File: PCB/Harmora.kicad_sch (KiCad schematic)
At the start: 14 parts, among them U14 ATmega328p-AU, U17 128x64 2.42 inc, Y1 16Mhz

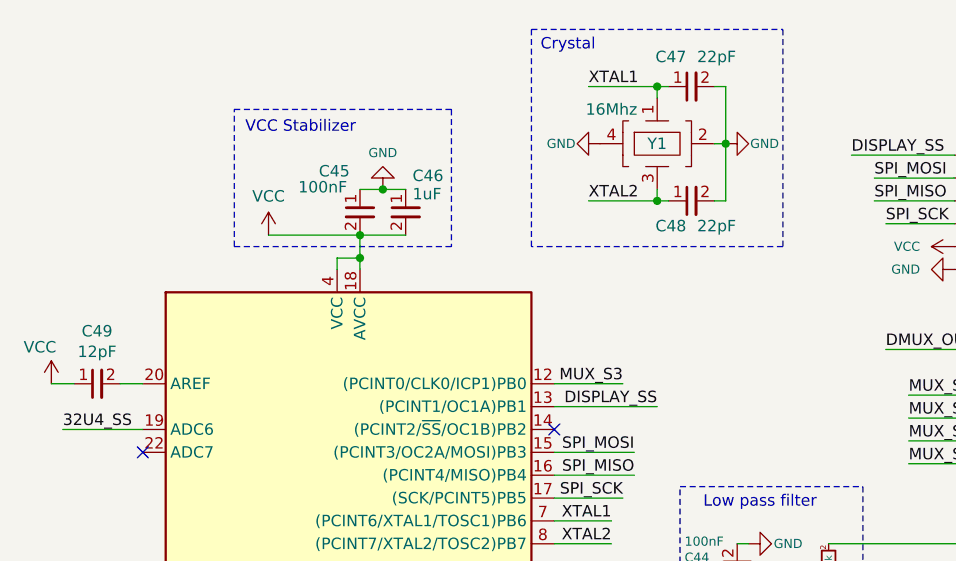
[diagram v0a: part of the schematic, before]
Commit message: new schematics
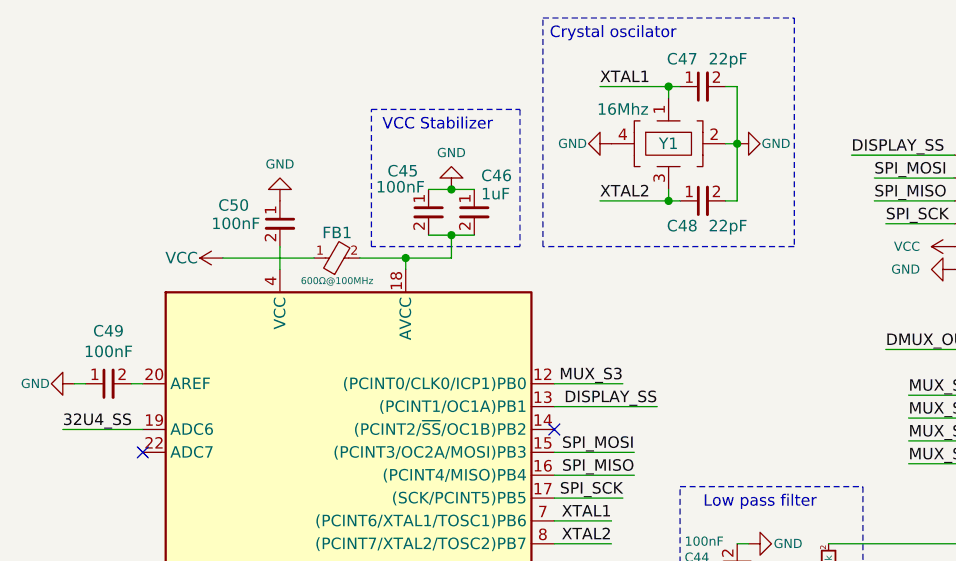
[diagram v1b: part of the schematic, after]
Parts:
- added C50: 100nF, Footprints:0603_C, symbol Symbols:Capacitor 0603
- added FB1: 600Ω@100MHz, Footprints:0603_FB, symbol Symbols:Ferrite_beat
- C44, C45, C46, C47, C48: footprint (none) -> Footprints:0603_C
- C49: value 12pF -> 100nF; footprint (none) -> Footprints:0603_C
- R10, R11, R12, R13, R9: footprint (none) -> Footprints:0603_R
- U14: footprint (none) -> Footprints:ATMEGA328P-AU
- U17: footprint (none) -> Footprints:SPI Screen PinHeader
- Y1: footprint (none) -> Footprints:Crystal Oscillator 16MHz
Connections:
- net GND: now also C49.1, C50.1
- net VCC: now also FB1.1; no longer C45.2, C46.2, C49.1, U14.18 (AVCC), U14.4 (VCC)
- new net: C45.2, C46.2, FB1.2, U14.18 (AVCC)
- new net: C50.2, U14.4 (VCC)
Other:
- sheet ATmega32u4: file MCU_32u4.kicad_sch -> schematic_pages/MCU_32u4.kicad_sch
- note added: "Crystal oscilator"
- note removed: "Crystal"
- moved on the sheet: C45, C46, C47, C48, C49, Y1
